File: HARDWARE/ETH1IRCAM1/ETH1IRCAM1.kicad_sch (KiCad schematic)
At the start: 8 parts

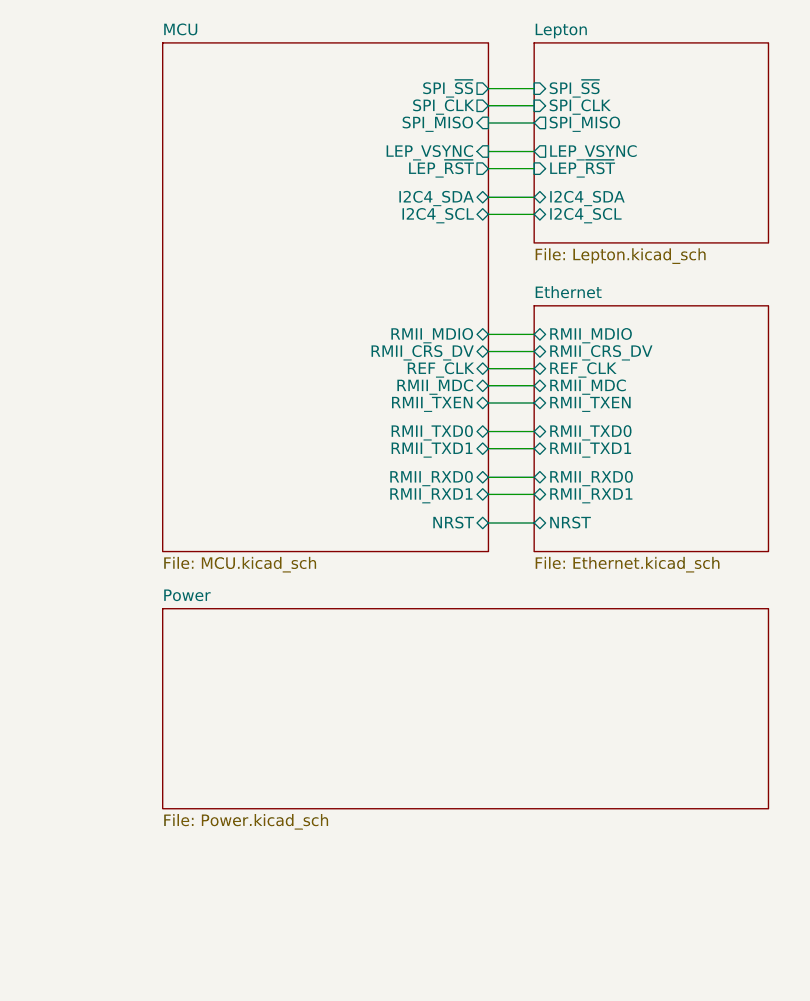
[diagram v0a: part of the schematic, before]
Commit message: Bug fixes
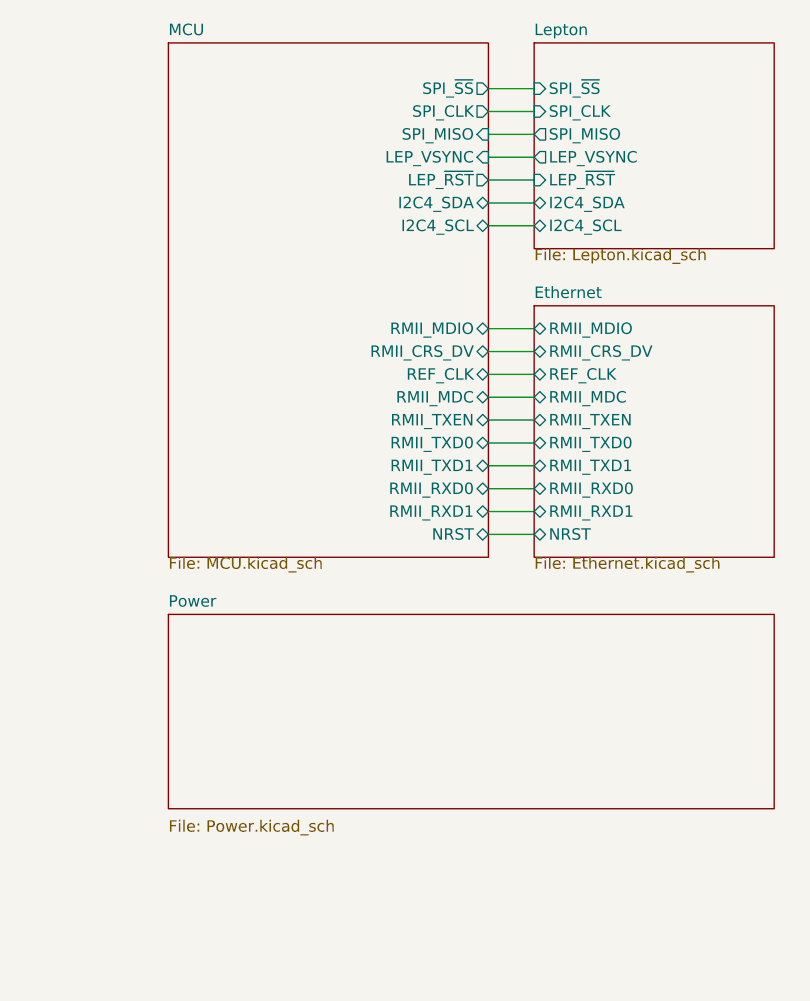
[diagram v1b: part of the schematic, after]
